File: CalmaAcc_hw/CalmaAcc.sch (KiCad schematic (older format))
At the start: 26 parts

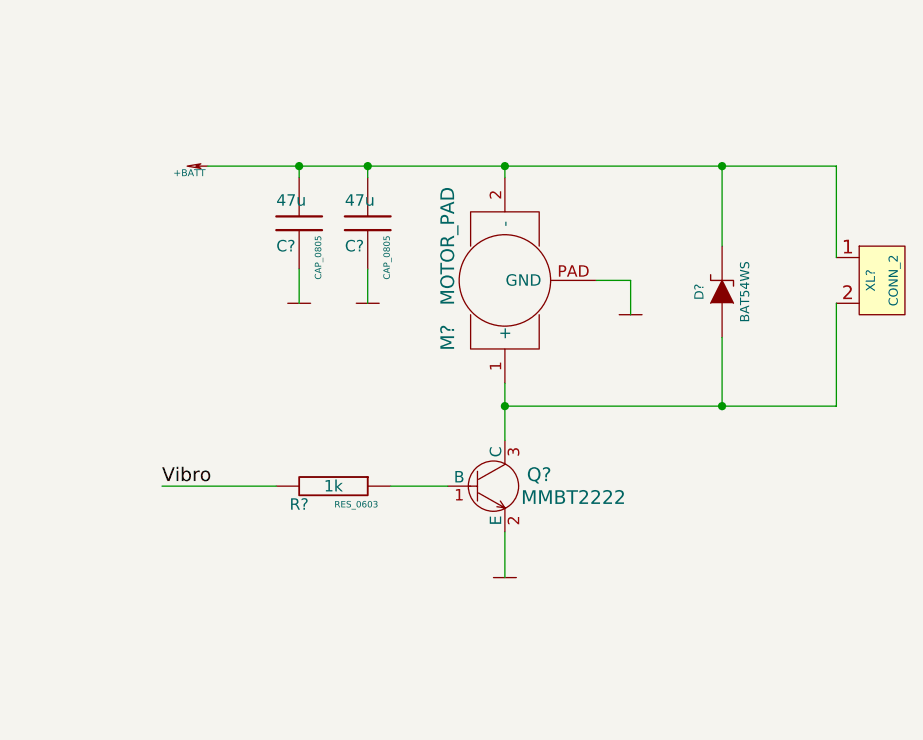
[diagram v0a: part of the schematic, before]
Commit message: scheme update
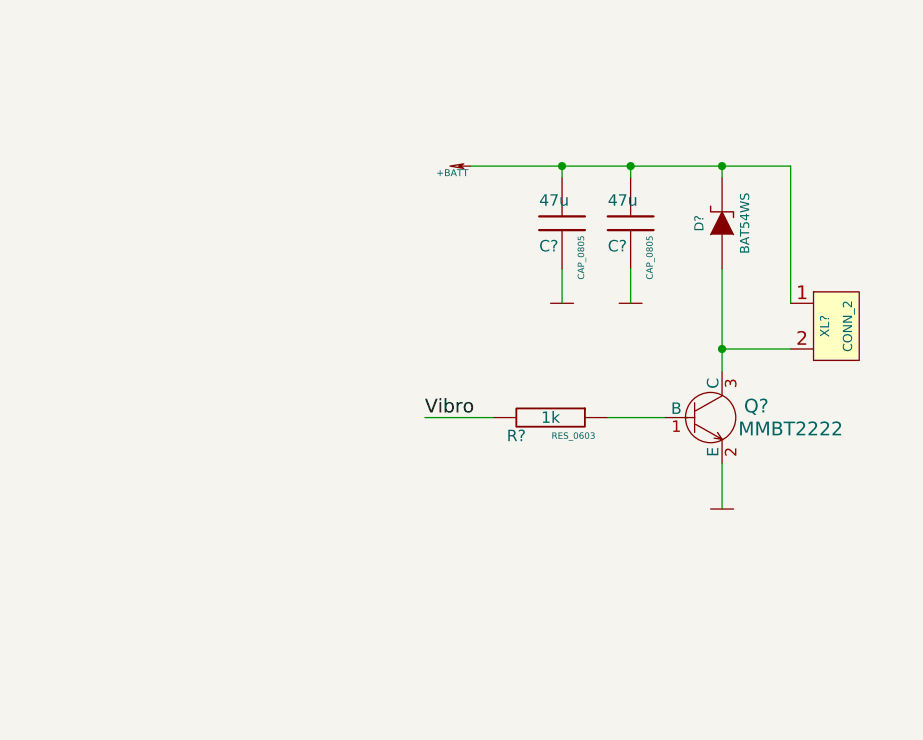
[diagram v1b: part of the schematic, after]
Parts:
- removed M?: MOTOR_PAD, symbol MOTOR_PAD
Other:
- moved on the sheet: C?, D?, Q?, R?, XL?
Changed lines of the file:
@@
 	-1   0    0    1
-$EndComp
-$Comp
-L MOTOR_PAD M?
-U 1 1 564889FE
-P 12800 6450
-F 0 "M?" H 12550 6700 60  0000 C CNN
-F 1 "MOTOR_PAD" H 12950 6700 60  0000 C CNN
-F 2 "" H 12800 6450 60  0000 C CNN
-F 3 "" H 12800 6450 60  0000 C CNN
-	1    12800 6450
-	0    -1   -1   0
-$EndComp
-$Comp
-L GND #PWR?
-U 1 1 56488A75
-P 13350 6600
-F 0 "#PWR?" H 13440 6580 30  0001 C CNN
-F 1 "GND" H 13350 6520 30  0001 C CNN
-F 2 "" H 13350 6600 60  0000 C CNN
-F 3 "" H 13350 6600 60  0000 C CNN
-	1    13350 6600
-	1    0    0    -1
 $EndComp
 Wire Wire Line
@@
 Wire Wire Line
 	8350 8450 8800 8450
-Wire Wire Line
-	13200 6450 13350 6450
-Wire Wire Line
-	13350 6450 13350 6600
 $Comp
 L C C?
 U 1 1 56488B03
-P 12200 6200
-F 0 "C?" H 12100 6100 50  0000 L CNN
-F 1 "47u" H 12100 6300 50  0000 L CNN
-F 2 "CAP_0805" V 12300 6050 28  0000 C BNN
-F 3 "" H 12200 6200 60  0000 C CNN
-	1    12200 6200
+P 13350 6200
+F 0 "C?" H 13250 6100 50  0000 L CNN
+F 1 "47u" H 13250 6300 50  0000 L CNN
+F 2 "CAP_0805" V 13450 6050 28  0000 C BNN
+F 3 "" H 13350 6200 60  0000 C CNN
+	1    13350 6200
 	1    0    0    -1
 $EndComp
@@
 L C C?
 U 1 1 56488B5E
-P 11900 6200
-F 0 "C?" H 11800 6100 50  0000 L CNN
-F 1 "47u" H 11800 6300 50  0000 L CNN
-F 2 "CAP_0805" V 12000 6050 28  0000 C BNN
-F 3 "" H 11900 6200 60  0000 C CNN
-	1    11900 6200
+P 13050 6200
+F 0 "C?" H 12950 6100 50  0000 L CNN
+F 1 "47u" H 12950 6300 50  0000 L CNN
+F 2 "CAP_0805" V 13150 6050 28  0000 C BNN
+F 3 "" H 13050 6200 60  0000 C CNN
+	1    13050 6200
 	1    0    0    -1
 $EndComp
@@
 L +BATT #PWR?
 U 1 1 56488C25
-P 11500 5950
-F 0 "#PWR?" H 11500 5910 30  0001 C CNN
-F 1 "+BATT" H 11580 5980 30  0000 C CNN
-F 2 "" H 11500 5950 60  0000 C CNN
-F 3 "" H 11500 5950 60  0000 C CNN
-	1    11500 5950
+P 12650 5950
+F 0 "#PWR?" H 12650 5910 30  0001 C CNN
+F 1 "+BATT" H 12730 5980 30  0000 C CNN
+F 2 "" H 12650 5950 60  0000 C CNN
+F 3 "" H 12650 5950 60  0000 C CNN
+	1    12650 5950
 	-1   0    0    1
 $EndComp
@@
 L D_Shottky D?
 U 1 1 56488C75
-P 13750 6500
-F 0 "D?" H 13750 6600 40  0000 C CNN
-F 1 "BAT54WS" H 13750 6400 40  0000 C CNN
-F 2 "" H 13750 6500 60  0000 C CNN
-F 3 "" H 13750 6500 60  0000 C CNN
-	1    13750 6500
+P 13750 6200
+F 0 "D?" H 13750 6300 40  0000 C CNN
+F 1 "BAT54WS" H 13750 6100 40  0000 C CNN
+F 2 "" H 13750 6200 60  0000 C CNN
+F 3 "" H 13750 6200 60  0000 C CNN
+	1    13750 6200
 	0    -1   -1   0
 $EndComp
@@
 L CONN_2 XL?
 U 1 1 56488D61
-P 14450 6450
-F 0 "XL?" V 14400 6450 40  0000 C CNN
-F 1 "CONN_2" V 14500 6450 40  0000 C CNN
-F 2 "" H 14450 6450 60  0000 C CNN
-F 3 "" H 14450 6450 60  0000 C CNN
-	1    14450 6450
-	1    0    0    -1
-$EndComp
-Wire Wire Line
-	12800 6000 12800 5950
-Wire Wire Line
-	11500 5950 14250 5950
-Wire Wire Line
-	11900 6000 11900 5950
-Connection ~ 11900 5950
-Wire Wire Line
-	12200 6000 12200 5950
-Connection ~ 12200 5950
-Wire Wire Line
-	13750 5950 13750 6300
-Connection ~ 12800 5950
-Wire Wire Line
-	14250 5950 14250 6350
-Connection ~ 13750 5950
+P 14250 6650
+F 0 "XL?" V 14200 6650 40  0000 C CNN
+F 1 "CONN_2" V 14300 6650 40  0000 C CNN
+F 2 "" H 14250 6650 60  0000 C CNN
+F 3 "" H 14250 6650 60  0000 C CNN
+	1    14250 6650
+	1    0    0    -1
+$EndComp
+Wire Wire Line
+	13050 6000 13050 5950
+Connection ~ 13050 5950
+Wire Wire Line
+	13350 5950 13350 6000
 $Comp
 L GND #PWR?
 U 1 1 56488E9B
-P 12200 6550
-F 0 "#PWR?" H 12290 6530 30  0001 C CNN
-F 1 "GND" H 12200 6470 30  0001 C CNN
-F 2 "" H 12200 6550 60  0000 C CNN
-F 3 "" H 12200 6550 60  0000 C CNN
-	1    12200 6550
+P 13350 6550
+F 0 "#PWR?" H 13440 6530 30  0001 C CNN
+F 1 "GND" H 13350 6470 30  0001 C CNN
+F 2 "" H 13350 6550 60  0000 C CNN
+F 3 "" H 13350 6550 60  0000 C CNN
+	1    13350 6550
 	1    0    0    -1
 $EndComp
@@
 L GND #PWR?
 U 1 1 56488EC7
-P 11900 6550
-F 0 "#PWR?" H 11990 6530 30  0001 C CNN
-F 1 "GND" H 11900 6470 30  0001 C CNN
-F 2 "" H 11900 6550 60  0000 C CNN
-F 3 "" H 11900 6550 60  0000 C CNN
-	1    11900 6550
-	1    0    0    -1
-$EndComp
-Wire Wire Line
-	12200 6400 12200 6550
-Wire Wire Line
-	11900 6400 11900 6550
+P 13050 6550
+F 0 "#PWR?" H 13140 6530 30  0001 C CNN
+F 1 "GND" H 13050 6470 30  0001 C CNN
+F 2 "" H 13050 6550 60  0000 C CNN
+F 3 "" H 13050 6550 60  0000 C CNN
+	1    13050 6550
+	1    0    0    -1
+$EndComp
+Wire Wire Line
+	13350 6400 13350 6550
+Wire Wire Line
+	13050 6400 13050 6550
 $Comp
 L NPN Q?
 U 1 1 56488F54
-P 12750 7350
-F 0 "Q?" H 12950 7400 60  0000 C CNN
-F 1 "MMBT2222" H 13100 7300 60  0000 C CNN
-F 2 "" H 12750 7350 60  0000 C CNN
-F 3 "" H 12750 7350 60  0000 C CNN
-	1    12750 7350
+P 13700 7050
+F 0 "Q?" H 13900 7100 60  0000 C CNN
+F 1 "MMBT2222" H 14050 7000 60  0000 C CNN
+F 2 "" H 13700 7050 60  0000 C CNN
+F 3 "" H 13700 7050 60  0000 C CNN
+	1    13700 7050
 	1    0    0    -1
 $EndComp
@@
 L GND #PWR?
 U 1 1 56489007
-P 12800 7750
-F 0 "#PWR?" H 12890 7730 30  0001 C CNN
-F 1 "GND" H 12800 7670 30  0001 C CNN
-F 2 "" H 12800 7750 60  0000 C CNN
-F 3 "" H 12800 7750 60  0000 C CNN
-	1    12800 7750
-	1    0    0    -1
-$EndComp
-Wire Wire Line
-	12800 7550 12800 7750
-Wire Wire Line
-	12800 6900 12800 7150
-Wire Wire Line
-	13750 6700 13750 7000
-Wire Wire Line
-	12800 7000 14250 7000
-Connection ~ 12800 7000
-Wire Wire Line
-	14250 7000 14250 6550
-Connection ~ 13750 7000
+P 13750 7450
+F 0 "#PWR?" H 13840 7430 30  0001 C CNN
+F 1 "GND" H 13750 7370 30  0001 C CNN
+F 2 "" H 13750 7450 60  0000 C CNN
+F 3 "" H 13750 7450 60  0000 C CNN
+	1    13750 7450
+	1    0    0    -1
+$EndComp
+Wire Wire Line
+	13750 7250 13750 7450
 $Comp
 L R R?
 U 1 1 5648910B
-P 12050 7350
-F 0 "R?" V 12130 7200 50  0000 C CNN
-F 1 "1k" V 12050 7350 50  0000 C CNN
-F 2 "RES_0603" V 12130 7450 28  0000 C CNN
-F 3 "" H 12050 7350 60  0000 C CNN
-	1    12050 7350
-	0    1    1    0
-$EndComp
-Wire Wire Line
-	12550 7350 12300 7350
-Wire Wire Line
-	11800 7350 11300 7350
-Text Label 11300 7350 0    60   ~ 0
+P 13000 7050
+F 0 "R?" V 13080 6900 50  0000 C CNN
+F 1 "1k" V 13000 7050 50  0000 C CNN
+F 2 "RES_0603" V 13080 7150 28  0000 C CNN
+F 3 "" H 13000 7050 60  0000 C CNN
+	1    13000 7050
+	0    1    1    0
+$EndComp
+Wire Wire Line
+	13500 7050 13250 7050
+Text Label 12450 7050 0    60   ~ 0
 Vibro
 Text Label 10450 2250 2    60   ~ 0
@@
 Wire Wire Line
 	6100 1850 6300 1850
+Connection ~ 13350 5950
+Wire Wire Line
+	13750 5950 13750 6000
+Connection ~ 13750 5950
+Wire Wire Line
+	12750 7050 12450 7050
+Wire Wire Line
+	12650 5950 14050 5950
+Wire Wire Line
+	14050 5950 14050 6550
+Wire Wire Line
+	14050 6750 13750 6750
+Wire Wire Line
+	13750 6400 13750 6850
+Connection ~ 13750 6750
 $EndSCHEMATC
